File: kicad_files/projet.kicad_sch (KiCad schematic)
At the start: 63 parts, among them J1 STLink V3, J4 USB_B_Micro, J5 Conn_01x04, J6 Conn_01x02, Q1 BC817, Q2 BC817, Q3 NMOS, Q4 PMOS, Q5 BC817, Q6 BC817, SW2 Reset, SW3 SW_Omron_B3FS, SW4 SW_Omron_B3FS, SW5 SW_Omron_B3FS, U1 STM32G031K8Tx, U2 MCP4901, U3 LM1117MP-3.3, U4 TLV2372, U5 CD4066BM, U6 MCP4131, U7 MCP4131

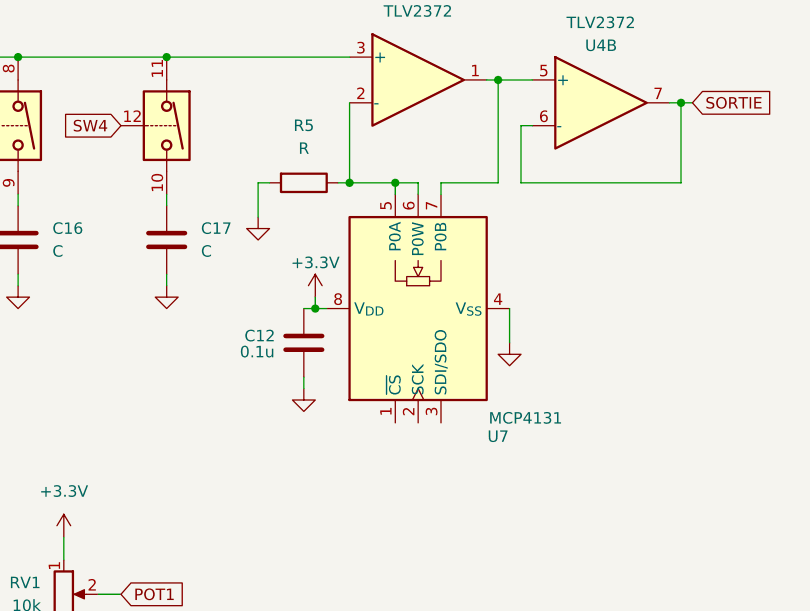
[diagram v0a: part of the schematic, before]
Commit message: simulation ok
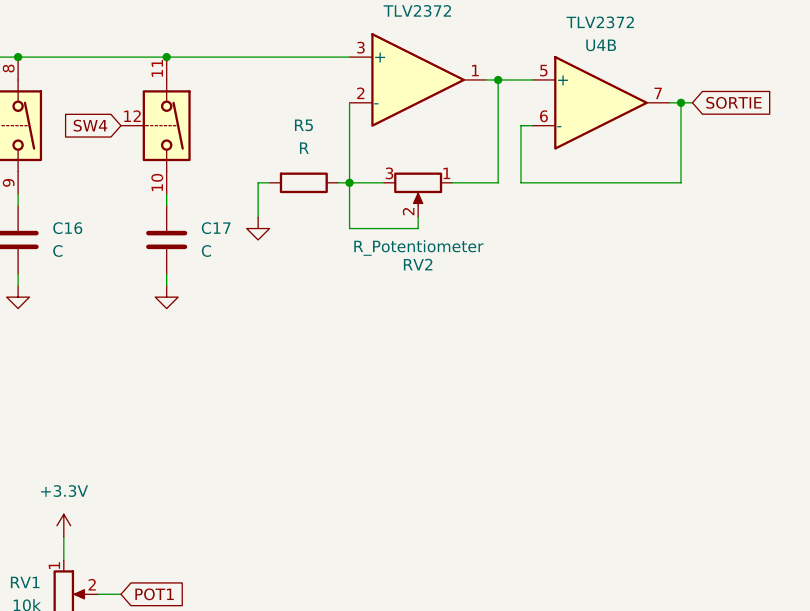
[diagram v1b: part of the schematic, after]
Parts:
- removed C12: 0.1u, symbol Device:C
- removed U7: MCP4131, Package_DIP:DIP-8_W7.62mm, symbol Potentiometer_Digital:MCP4131-xxxx-P
- added RV2: R_Potentiometer, symbol Device:R_Potentiometer
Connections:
- net at R5.1, U4.2 (-): now also RV2.2, RV2.3
- net at U4.1, U4.5 (+): now also RV2.1

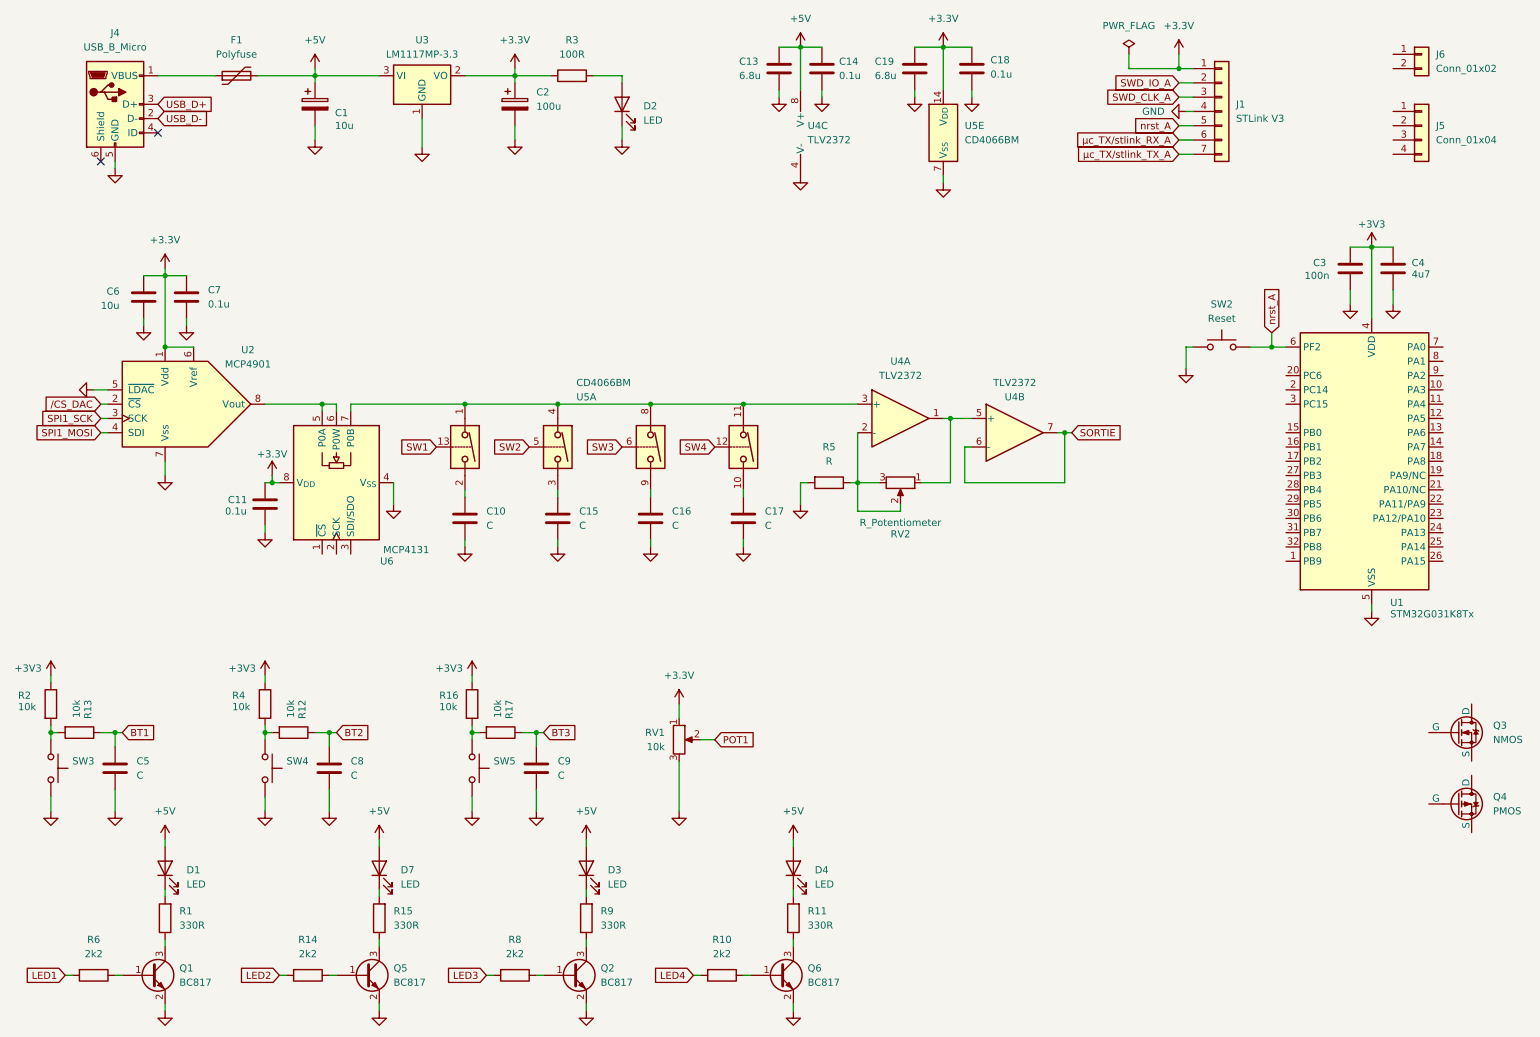
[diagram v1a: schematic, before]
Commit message: circuit kicad
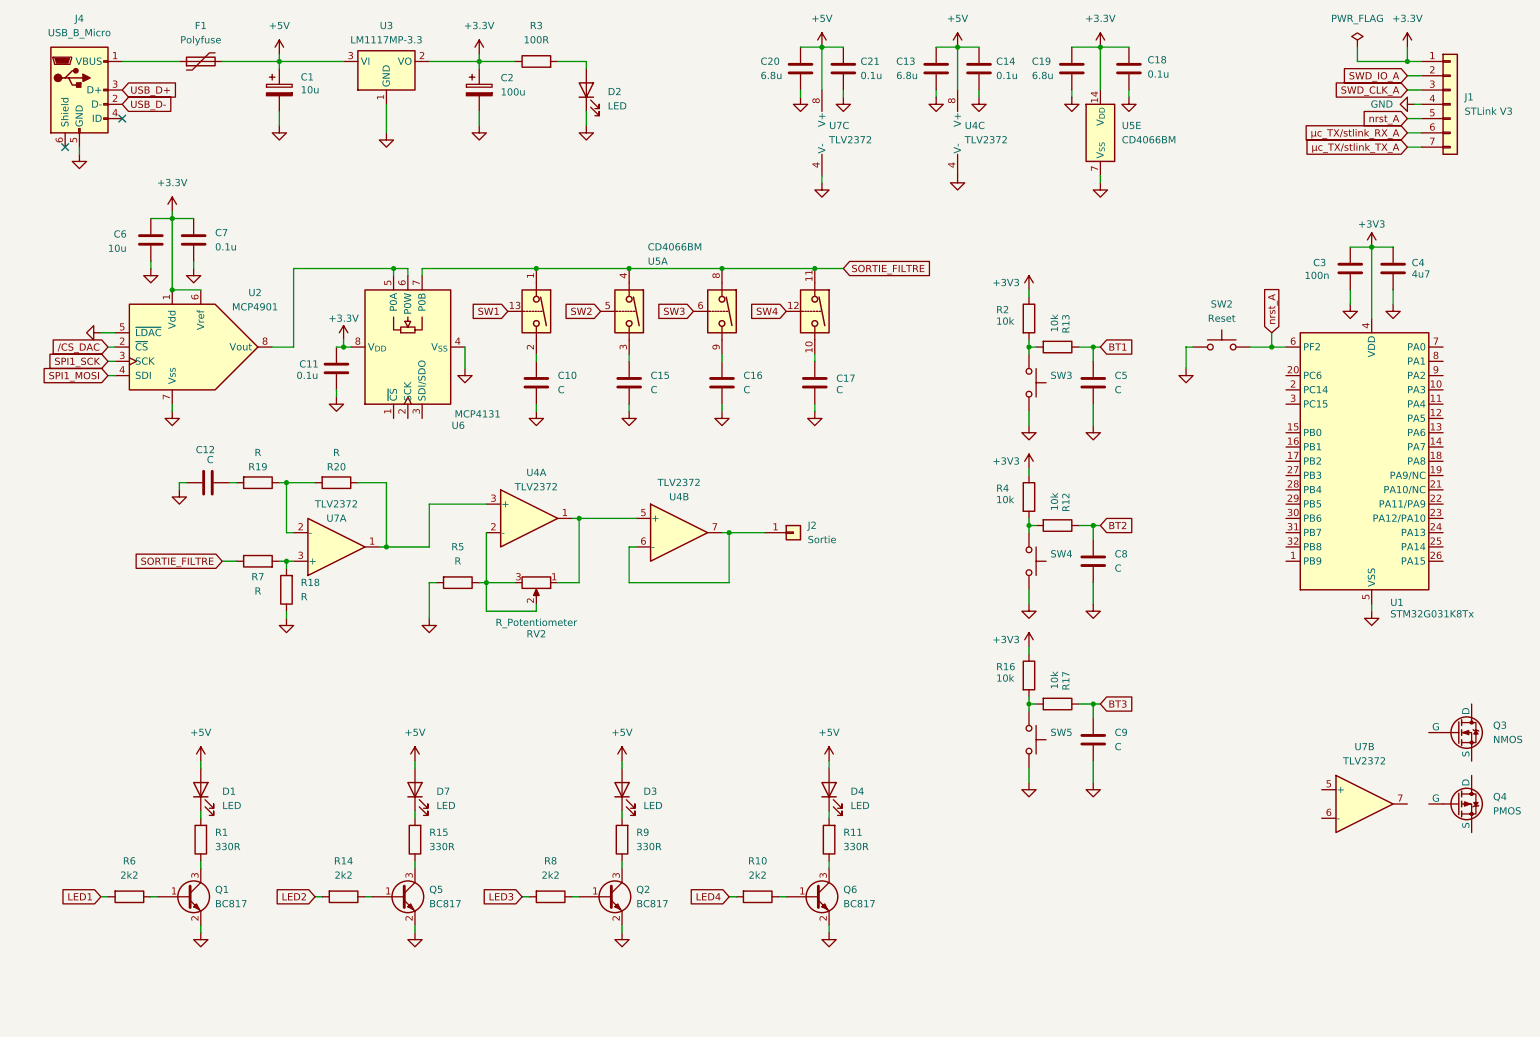
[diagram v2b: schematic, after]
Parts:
- removed J5: Conn_01x04, symbol Connector_Generic:Conn_01x04
- removed J6: Conn_01x02, symbol Connector_Generic:Conn_01x02
- removed RV1: 10k, symbol Device:R_Potentiometer
- added C12: C, symbol Device:C
- added C20: 6.8u, symbol Device:C
- added C21: 0.1u, symbol Device:C
- added J2: Sortie, symbol Connector_Generic:Conn_01x01
- added R18, R19, R20, R7: R, symbol Device:R
- added U7: TLV2372, symbol Amplifier_Operational:TLV2372
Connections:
- net +5V: now also C20.1, C21.1, U7.8 (V+)
- net SORTIE_FILTRE: now reaches U5.1, U5.11, U5.4, U5.8, U6.7 (P0B)
- net SORTIE_FILTRE: now also R7.1; no longer U4.3 (+)
- net SORTIE: no longer names the net of U4.6 (-), U4.7
- net SORTIE: now also J2.1 (Pin_1)
- new net: C12.1, R19.2
- new net: R20.1, U4.3 (+), U7.1
- new net: R18.2, R7.2, U7.3 (+)
- new net: R19.1, R20.2, U7.2 (-)
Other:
- moved on the sheet: C1, C10, C11, C13, C14, C15, C16, C17, C18, C19, C2, C5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
